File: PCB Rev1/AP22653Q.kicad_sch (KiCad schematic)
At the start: 5 parts, among them J4 MICRO_SD

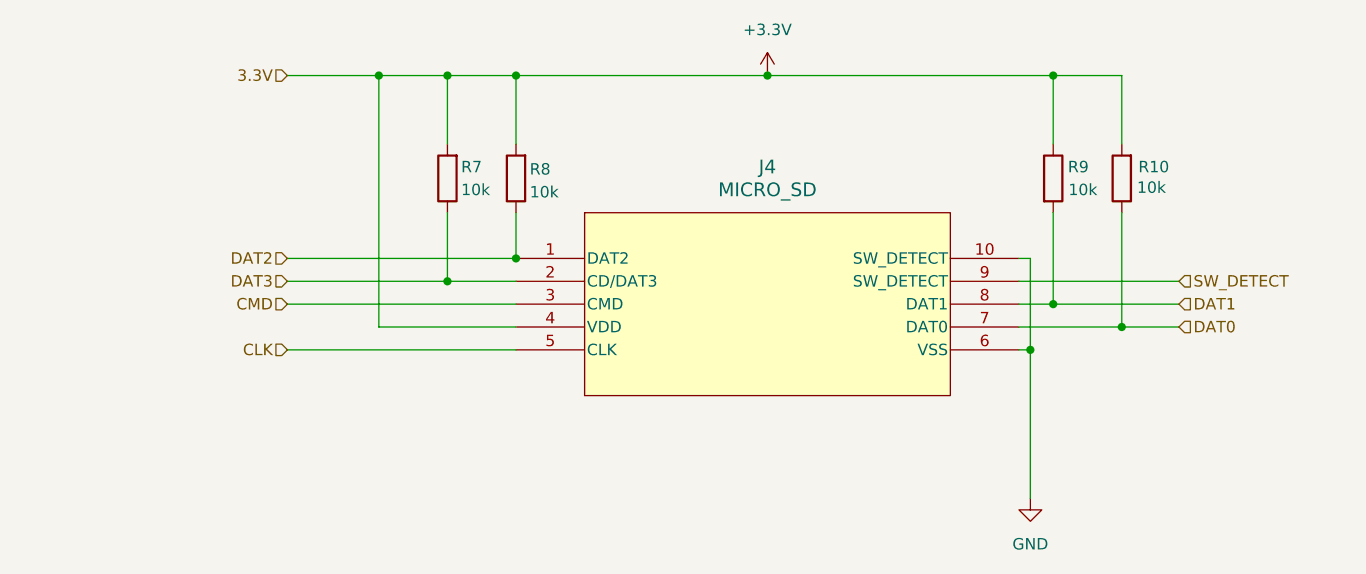
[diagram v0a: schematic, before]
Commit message: added new files and switches, notes,tps
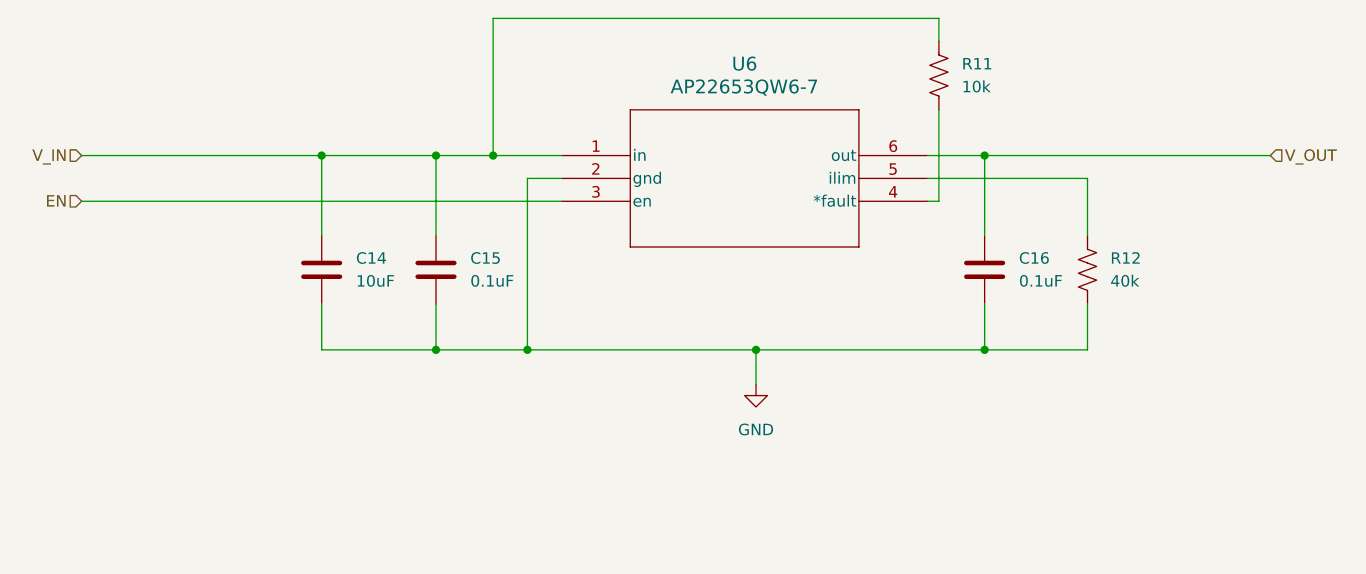
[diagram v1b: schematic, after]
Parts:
- removed J4: MICRO_SD, footprints:104031-0811_MOL, symbol sd_card_holder:1040310811
- removed R10, R7, R8, R9: 10k, symbol Device:R
- added C14: 10uF, symbol Device:C
- added C15, C16: 0.1uF, symbol Device:C
- added R11: 10k, symbol Device:R_US
- added R12: 40k, symbol Device:R_US
- added U6: AP22653QW6-7, footprints:SOT26-A1-AP22653Q_DIO, symbol voltage_switch:AP22653QW6-7
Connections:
- net GND: now also C14.2, C15.2, C16.2, R12.2, U6.2 (gnd)
- new net: R12.1, U6.5 (ilim)
- new net: R11.2, U6.4 (*fault)
- new net EN: U6.3 (en)
- new net V_IN: C14.1, C15.1, R11.1, U6.1 (in)
- new net V_OUT: C16.1, U6.6 (out)
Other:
- title: Micro SD Card -> Enable Switch for GPS and SD Card
